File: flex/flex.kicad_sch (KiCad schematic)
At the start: 4 parts, among them J1 Conn_01x20_Socket, J2 501461-0491

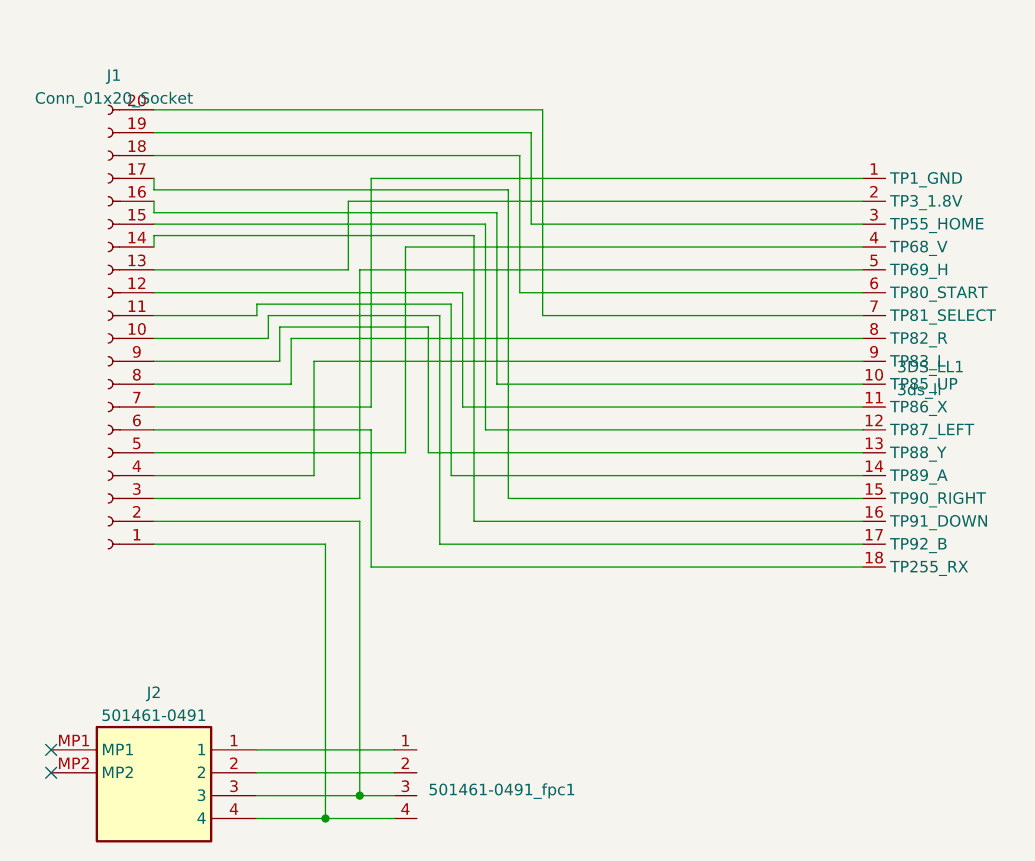
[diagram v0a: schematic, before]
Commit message: Add fpc
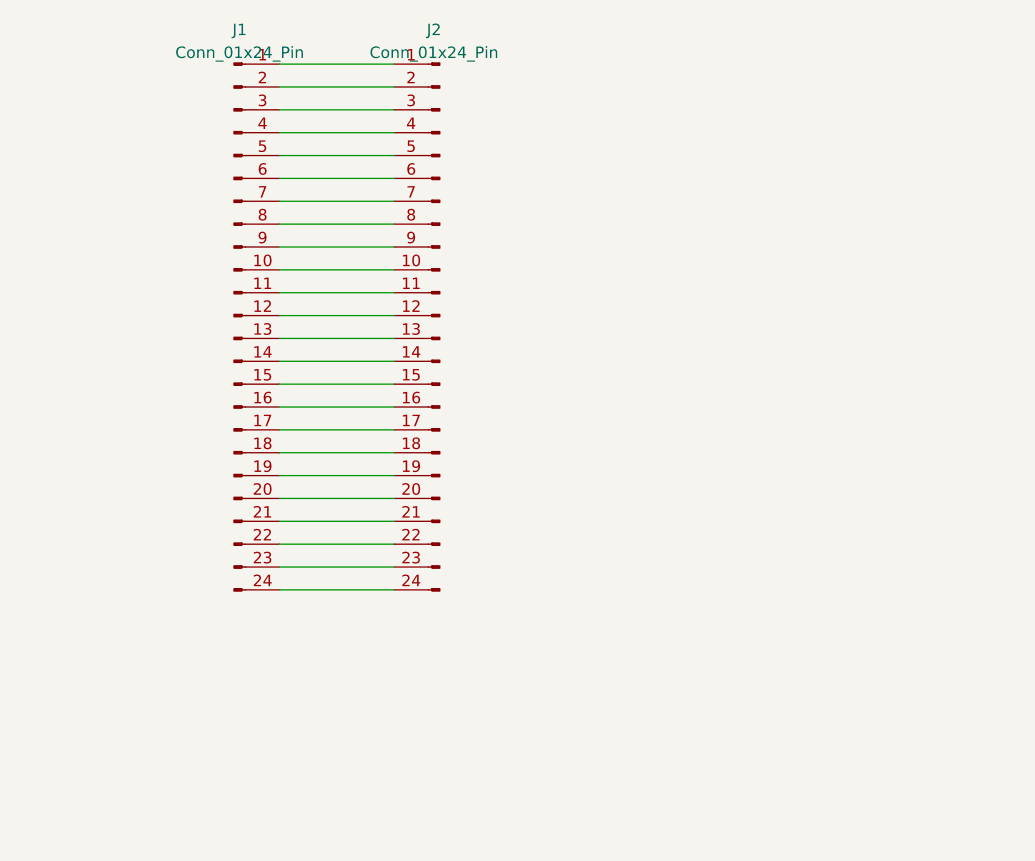
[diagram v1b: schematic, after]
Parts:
- removed 3DS_LL1: 3ds_ll, 3ds:3ds_ll, symbol 3ds:3ds_ll
- removed 501461-0491_fpc1: ~, 501461-0491_fpc:501461-0491_fpc, symbol 501461-0491_fpc:501461-0491_fpc
- removed J1: Conn_01x20_Socket, Connector_PinHeader_2.54mm:PinHeader_1x20_P2.54mm_Vertical, symbol Connector:Conn_01x20_Socket
- removed J2: 501461-0491, 501461-0491:5014610491, symbol 501461-0491:501461-0491
- added J1: Conn_01x24_Pin, lib:3ds_ll, symbol Connector:Conn_01x24_Pin
- added J2: Conn_01x24_Pin, lib:bss, symbol Connector:Conn_01x24_Pin
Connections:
- new net: J1.1 (Pin_1), J2.1 (Pin_1)
- new net: J1.10 (Pin_10), J2.10 (Pin_10)
- new net: J1.11 (Pin_11), J2.11 (Pin_11)
- new net: J1.12 (Pin_12), J2.12 (Pin_12)
- new net: J1.13 (Pin_13), J2.13 (Pin_13)
- new net: J1.14 (Pin_14), J2.14 (Pin_14)
- new net: J1.15 (Pin_15), J2.15 (Pin_15)
- new net: J1.16 (Pin_16), J2.16 (Pin_16)
- new net: J1.17 (Pin_17), J2.17 (Pin_17)
- new net: J1.18 (Pin_18), J2.18 (Pin_18)
- new net: J1.19 (Pin_19), J2.19 (Pin_19)
- new net: J1.2 (Pin_2), J2.2 (Pin_2)
- new net: J1.20 (Pin_20), J2.20 (Pin_20)
- new net: J1.21 (Pin_21), J2.21 (Pin_21)
- new net: J1.22 (Pin_22), J2.22 (Pin_22)
- new net: J1.23 (Pin_23), J2.23 (Pin_23)
- new net: J1.24 (Pin_24), J2.24 (Pin_24)
- new net: J1.3 (Pin_3), J2.3 (Pin_3)
- new net: J1.4 (Pin_4), J2.4 (Pin_4)
- new net: J1.5 (Pin_5), J2.5 (Pin_5)
- new net: J1.6 (Pin_6), J2.6 (Pin_6)
- new net: J1.7 (Pin_7), J2.7 (Pin_7)
- new net: J1.8 (Pin_8), J2.8 (Pin_8)
- new net: J1.9 (Pin_9), J2.9 (Pin_9)
- no-connect marks 2 -> 0
